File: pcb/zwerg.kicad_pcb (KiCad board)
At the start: 2 copper layers, 144.2 x 106.7 mm, 57 parts, among them J1 AudioJack4, U1 RP2040-Matrix

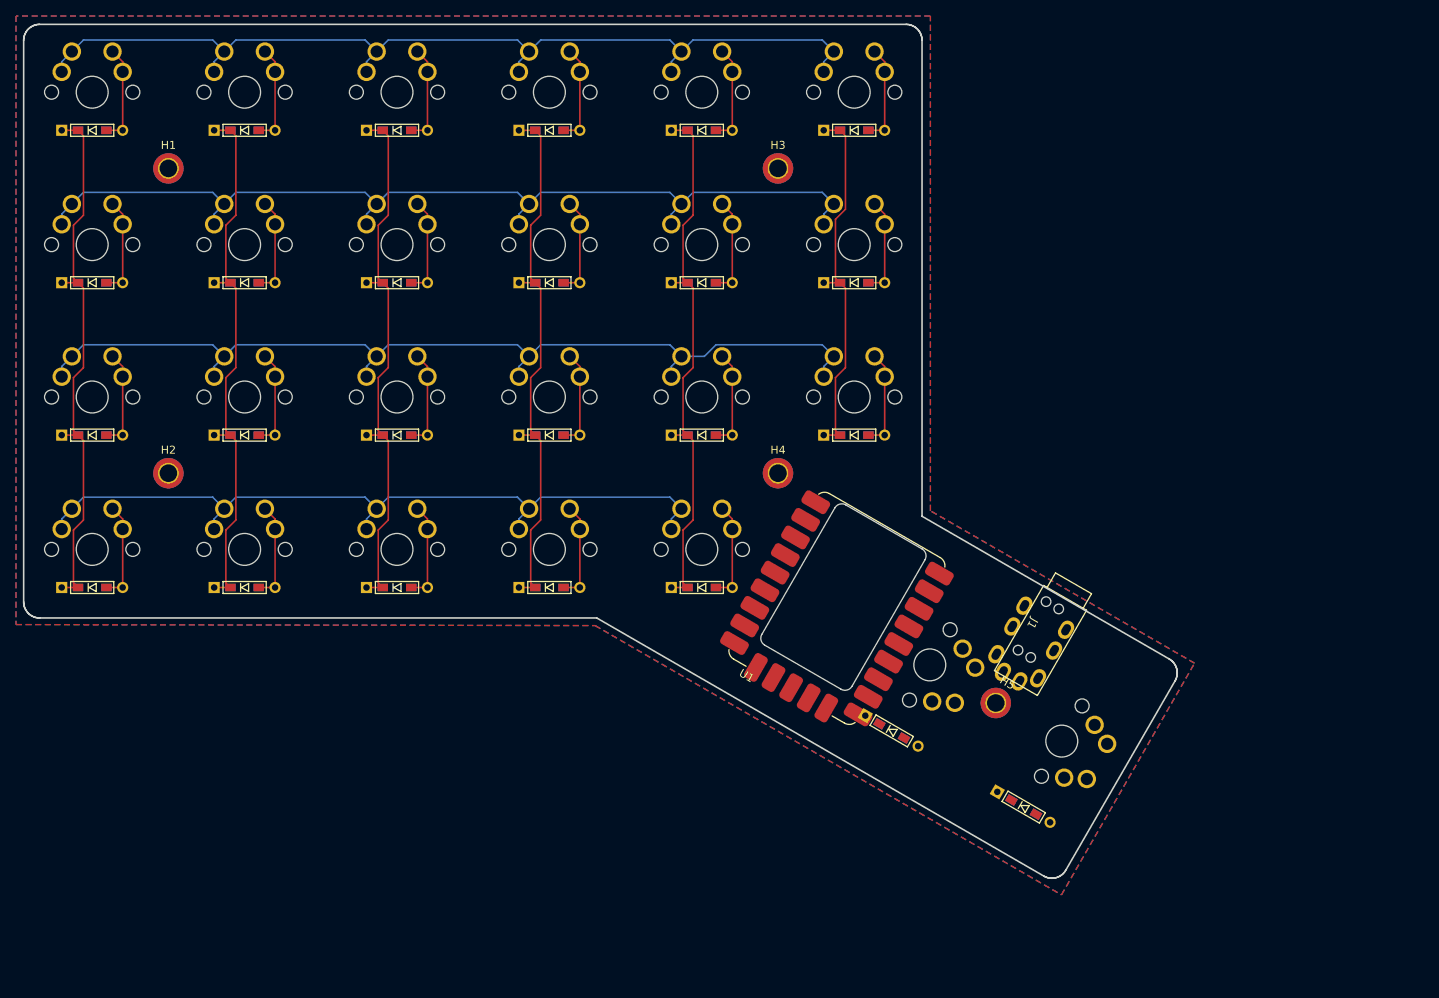
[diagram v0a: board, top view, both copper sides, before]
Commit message: updated pcb and case v1.0
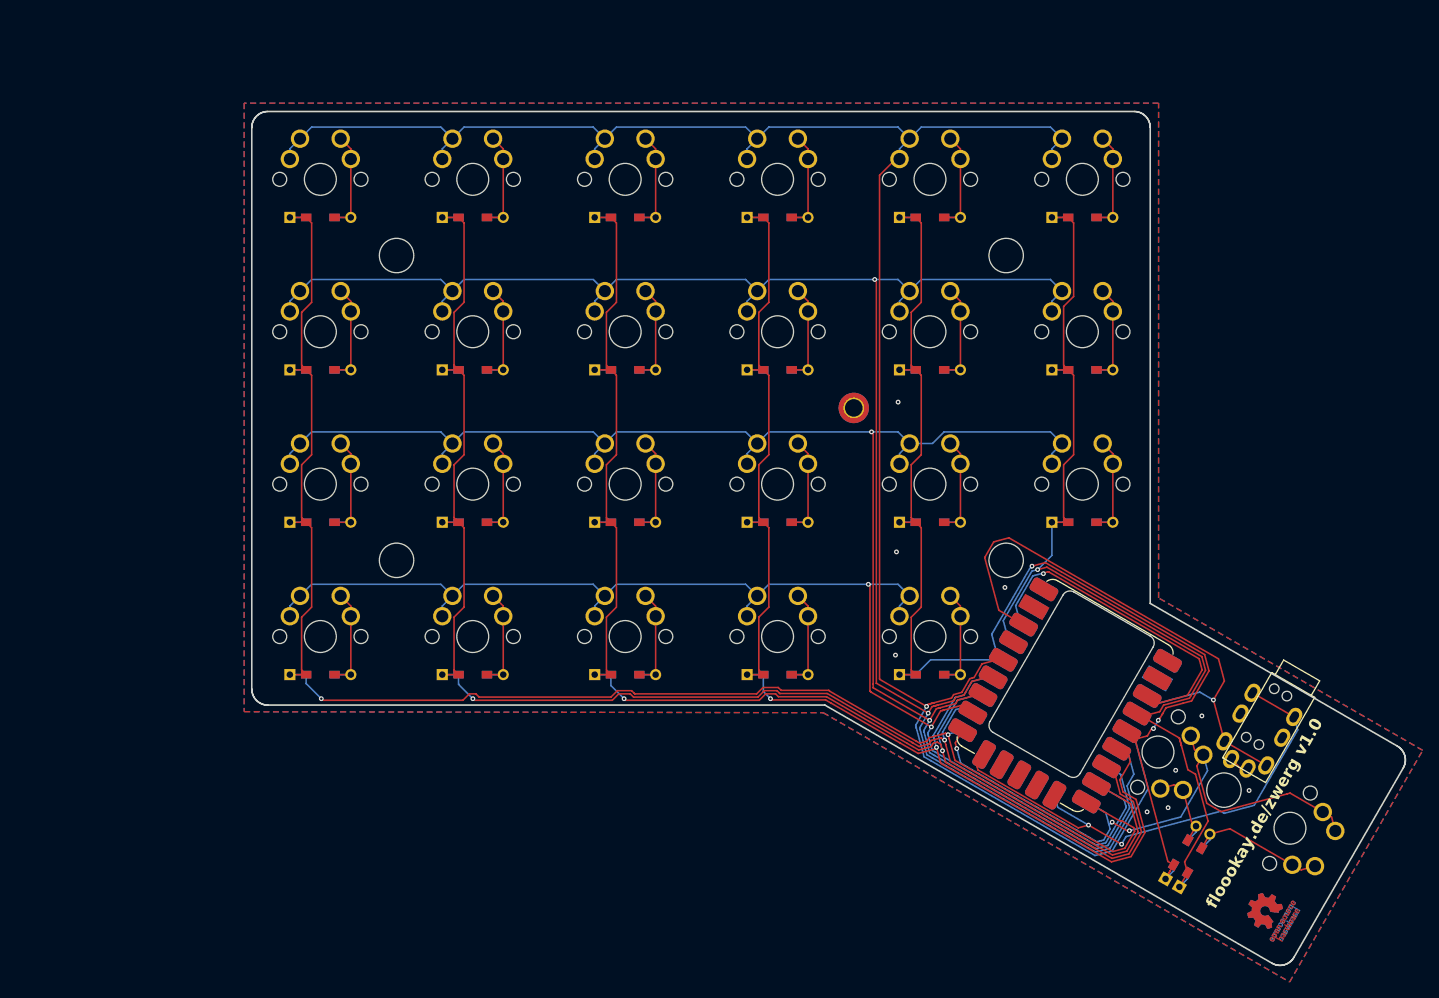
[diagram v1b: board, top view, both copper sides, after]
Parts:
- added H6: MountingHole, MountingHole:MountingHole_2.2mm_M2_DIN965_Pad_TopBottom, F.Cu at (152.3, 87.1)
- added REF**: OSHW-Logo_5.7x6mm_Copper, Symbol:OSHW-Logo_5.7x6mm_Copper, F.Cu at (204.4, 150.4)
- added REF**: OSHW-Logo_5.7x6mm_Copper, Symbol:OSHW-Logo_5.7x6mm_Copper, B.Cu at (204.4, 150.4)
- D1, D10, D11, D12, D13, D14, D15, D16, D17, D18, D19, D2, D20, D21, D22, D23, D24, D25, D3, D4, D5, D6, D7, D8, D9: footprint kbd:D3_TH_SMD -> zwerg:D3_TH_SMD
- H1, H2, H3, H4, H5: footprint MountingHole:MountingHole_2.2mm_M2_DIN965_Pad_TopBottom -> MountingHole:MountingHole_4.3mm_M4
- U1: footprint PCM_marbastlib-xp-promicroish:RP2040-Matrix_AC -> zwerg:RP2040-Matrix_fb
- moved D21 39.2 mm to (193.2, 142.7), turned to 60 degrees
- moved D3 30.5 mm to (85.7, 101.4)
- moved D4 30.5 mm to (85.7, 120.4)
- moved D8 30.5 mm to (104.7, 120.4)
- moved H2 30.5 mm to (95.2, 106.1)
- moved MX3 30.5 mm to (85.7, 96.6)
- moved MX4 30.5 mm to (85.7, 115.7)
- moved MX7 30.5 mm to (104.7, 96.6)
- moved D7 30.5 mm to (104.7, 101.4)
- moved MX8 30.5 mm to (104.7, 115.7)
- moved MX1 30.5 mm to (85.7, 58.5)
- moved MX2 30.5 mm to (85.7, 77.6)
- moved D1 30.5 mm to (85.7, 63.3)
- moved D2 30.5 mm to (85.7, 82.3)
- moved H1 30.5 mm to (95.2, 68.0)
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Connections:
- J1 pad T: tx -> unconnected-(J1-PadT)
- U1 pad 20: tx -> unconnected-(U1-P12-Pad20)
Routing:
- net row0: track 119.7 -> 256.4 mm, vias 0 -> 1
- net col0: track 68.4 -> 202.1 mm, vias 0 -> 2
- net col1: track 68.4 -> 189.1 mm, vias 0 -> 2
- net row1: track 119.7 -> 234.6 mm, vias 0 -> 2
- net col2: track 68.4 -> 174.6 mm, vias 0 -> 2
- net col4: track 68.4 -> 167.3 mm, vias 0 -> 3
- net col3: track 68.4 -> 161.6 mm, vias 0 -> 2
- net col5: track 46.3 -> 136.7 mm, vias 0 -> 1
- net row2: track 119.7 -> 209.8 mm, vias 0 -> 2
- net row4: track 0.00 -> 78.2 mm, vias 0 -> 3
- net vcc: track 0.00 -> 70.8 mm, vias 0 -> 1
- net row3: track 96.3 -> 163.6 mm, vias 0 -> 2
- net rx: track 0.00 -> 66.6 mm, vias 0 -> 2
- net unconnected-(U1-P2-Pad12): track 0.00 -> 41.3 mm, vias 0 -> 1
- net Net-(D22-A): track 0.00 -> 18.9 mm
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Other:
- board text added: "floookay.de/zwerg v1.0"
